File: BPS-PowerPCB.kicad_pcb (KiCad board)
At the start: 2 copper layers, 5 parts, among them J1 Conn_01x02, J2 Conn_01x02, J3 Conn_01x02, J4 Conn_01x02, J5 Conn_01x02

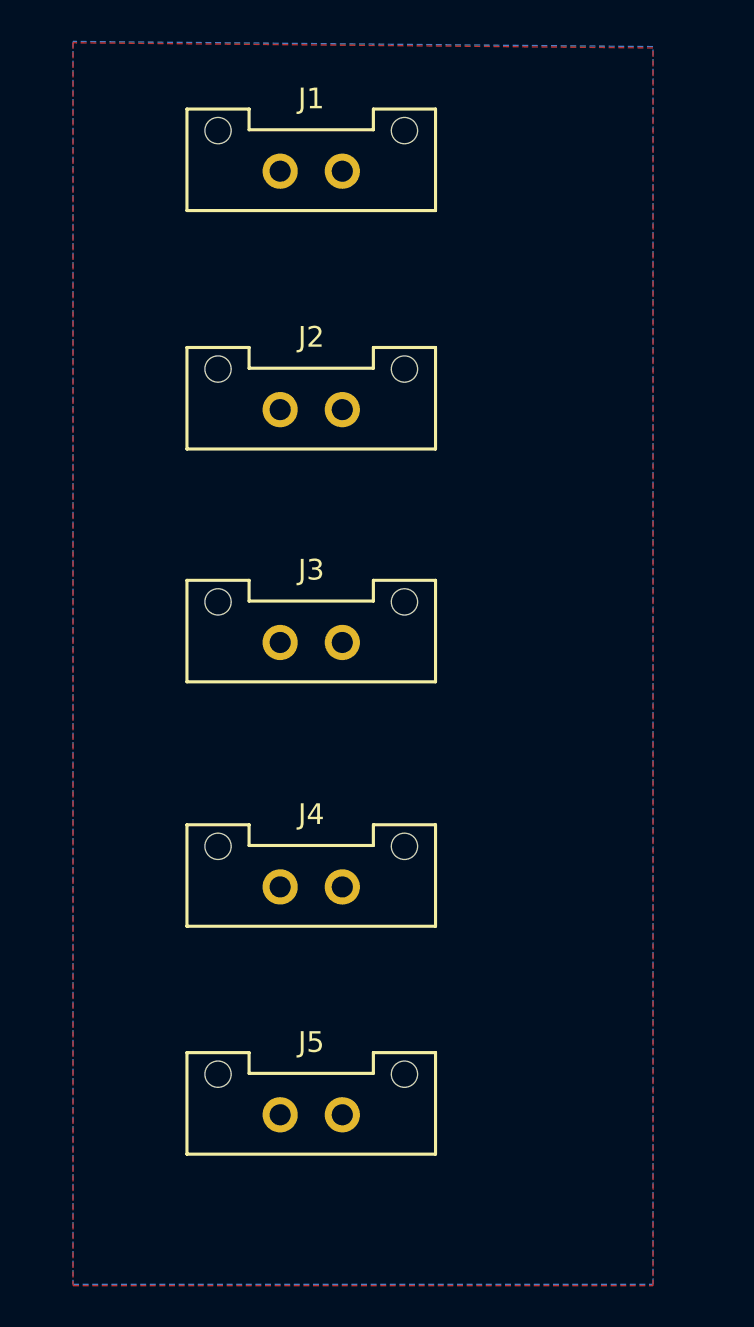
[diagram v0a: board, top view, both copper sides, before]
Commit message: done may need to add labels
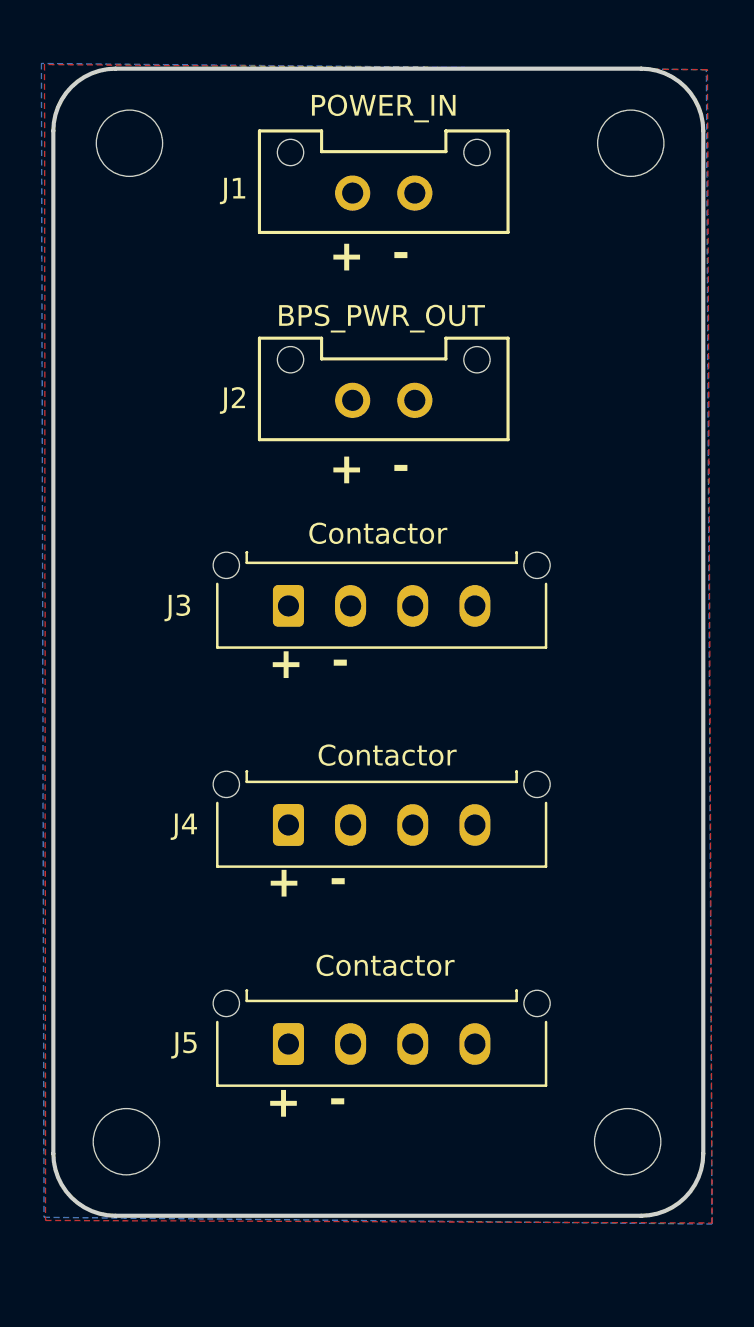
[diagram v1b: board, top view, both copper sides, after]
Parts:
- added REF**: MountingHole_3.2mm_M3, MountingHole:MountingHole_3.2mm_M3, F.Cu at (131.0, 75.8)
- added REF**: MountingHole_3.2mm_M3, MountingHole:MountingHole_3.2mm_M3, F.Cu at (155.2, 75.8)
- added REF**: MountingHole_3.2mm_M3, MountingHole:MountingHole_3.2mm_M3, F.Cu at (130.8, 124.0)
- added REF**: MountingHole_3.2mm_M3, MountingHole:MountingHole_3.2mm_M3, F.Cu at (155.0, 124.0)
- J1: value Conn_01x02 -> POWER_IN
- J2: value Conn_01x02 -> BPS_PWR_OUT
- J3, J4, J5: value Conn_01x02 -> Contactor; footprint UTSVT_Connectors:Molex_MicroFit3.0_1x2xP3.00mm_PolarizingPeg_Vertical -> Connector_Molex:Molex_Micro-Fit_3.0_43650-0415_1x04_P3.00mm_Vertical
- moved J1 3.66 mm to (141.8, 78.3)
- moved J2 3.53 mm to (141.8, 88.3)
- moved J5 3.44 mm to (138.7, 119.3)
- moved J4 3.02 mm to (138.7, 108.8)
- moved J3 1.81 mm to (138.7, 98.2)
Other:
- board outline added: 31.4 x 55.4 mm
- board text added: "+"
- board text added: "-"
